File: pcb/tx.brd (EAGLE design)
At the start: 28.1 x 45 mm, 37 parts, among them U3 MCP73831T-2ACI/OT, Y1 CRYSTAL-26MHZSMD-3.2X2.5

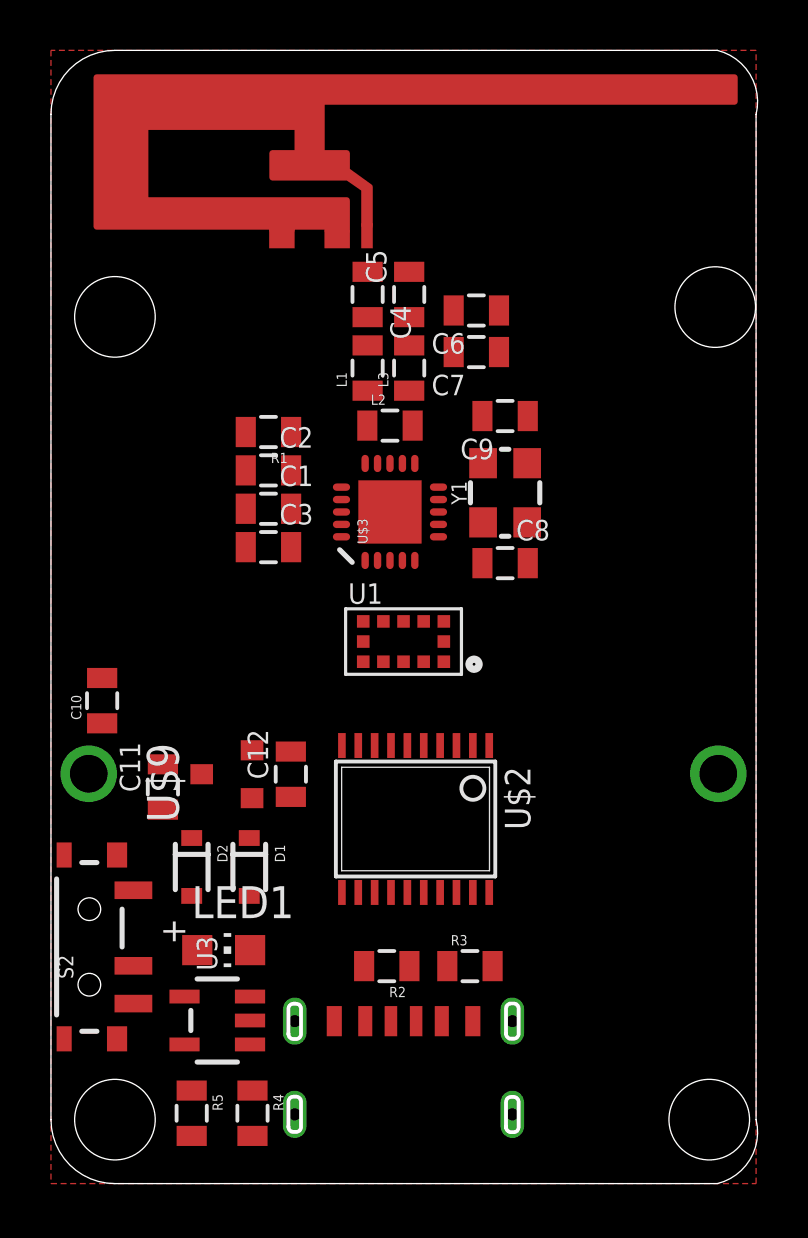
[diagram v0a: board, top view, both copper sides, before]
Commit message: tx before cleanup
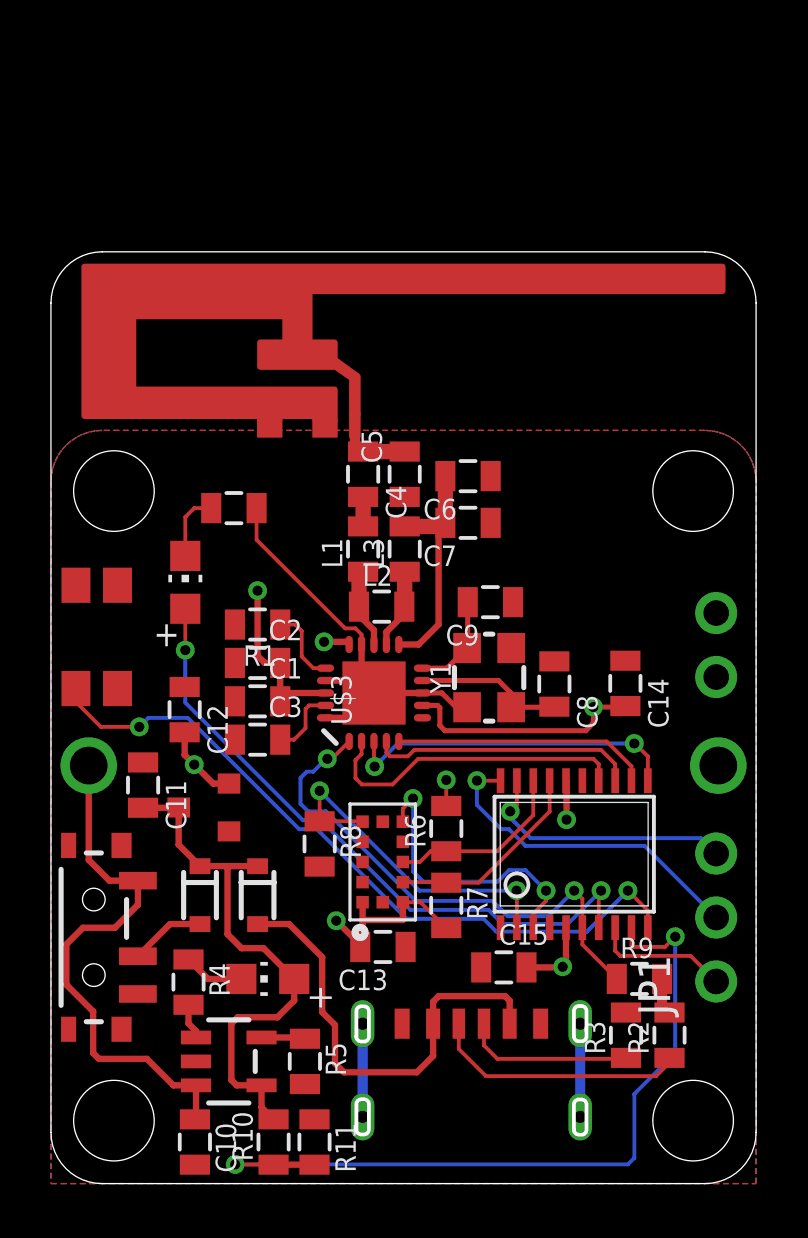
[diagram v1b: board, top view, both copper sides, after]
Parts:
- added 4K7, R9: 22K, joyAnalog:0805
- added C13: 100nF, clock:0805
- added C14, C15: 4.7uF, clock:0805
- added JP1: (no value), adafruit_changed:1X03-CLEANBIG
- added LED2: (no value), joyAnalog:CHIP-LED0805
- added R10, R11: 100K, SparkFun-Passives:0805
- added R6, R7, R8: 27K, SparkFun-Passives:0805
- added U$10: 324_SW, 3pos_slide_switch:342_SWICH_FOOT
- added U$11: PINHD1X2, adafruit_changed:1X02
- S2: device Adafruit Feather M0 Adalogger:SWITCH-SPST-SMD-A -> tx:SWITCH-SPST-SMD-A
- moved C10 17.9 mm to (5.71, 1.65), turned to 270 degrees
- moved R2 11.6 mm to (24.6, 5.89), turned to 90 degrees
- moved U1 8.79 mm to (13.2, 12.8), turned to 270 degrees
- moved C1 7.66 mm to (8.20, 19.2)
- moved C2 7.66 mm to (8.20, 20.7)
- moved C3 7.66 mm to (8.20, 17.6)
- moved R1 7.66 mm to (8.20, 22.2)
- moved U$4 7.53 mm to (9.85, 32.9)
- moved C9 7.41 mm to (17.4, 23.1)
- moved Y1 7.37 mm to (17.4, 20.1)
- moved U$6 7.36 mm to (25.5, 27.5)
- moved U$3 7.22 mm to (12.8, 19.5)
- moved L2 7.20 mm to (13.1, 22.9)
- moved L1 7.19 mm to (12.4, 25.2)
- moved L3 7.19 mm to (14.0, 25.2)
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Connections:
- removed net AVDD: U1.11
- removed net AVDDVCSEL: U1.1
- removed net AVSSVCSEL: U1.2
- new net N$18: R6.1, U$2.18, U1.9
- new net N$22: R7.1, U$2.17, U1.10
- new net N$23: R8.1, U$2.2, U1.5
- new net N$24: U$2.3, U1.7
- new net N$28: 4K7.2, LED2.C
- new net N$29: LED2.A, U$2.7
- new net N$30: U$10.P$2, U$2.10
- new net N$31: JP1.3, U$2.19
- new net N$32: JP1.2, U$2.20
- new net N$33: JP1.1, U$2.8
- new net N$35: R10.1, R11.2, U$2.9
- net +3V3: now also C13.1, C14.1, C15.1, R6.2, R7.2, U$11.1, U$2.16, U$2.5, U1.1, U1.11
- net GND: now also 4K7.1, C13.2, C14.2, C15.2, R11.1, R8.2, R9.2, S2.G1, S2.G2, S2.G3, S2.G4, U$10.P$4, U$11.2, U$2.1, U$2.15, U$4.GND, U$4.GND@1, U1.2
- net N$14: now also U$2.13
- net N$15: now also U$2.12
- net N$16: now also U$2.11
- net N$20: now also U$2.14
- net N$21: now also R9.1, U$2.6
- net N$27: now also R10.2
- net N$5: now also U$4.FEED
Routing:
- net +3V3: track 0.00 -> 34.2 mm, vias 0 -> 8
- net N$35: track 0.00 -> 31.2 mm, vias 0 -> 2
- net N$30: track 0.00 -> 29.0 mm, vias 0 -> 2
- net GND: track 0.00 -> 26.1 mm
- net N$29: track 0.00 -> 25.9 mm, vias 0 -> 2
- net N$27: track 0.00 -> 21.3 mm
- net N$25: track 0.00 -> 21.2 mm
- net N$21: track 0.00 -> 20.9 mm, vias 0 -> 2
- net N$26: track 0.00 -> 18.1 mm
- net N$23: track 0.00 -> 13.9 mm, vias 0 -> 2
- net N$16: track 0.00 -> 13.4 mm, vias 0 -> 2
- net N$32: track 0.00 -> 13.3 mm, vias 0 -> 1
- net N$20: track 0.00 -> 12.5 mm
- net N$24: track 0.00 -> 11.6 mm, vias 0 -> 2
- net N$14: track 0.00 -> 10.6 mm
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- added copper zone on layer 16, net +3V3
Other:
- board size 28.1 x 45 mm -> 28 x 37 mm
